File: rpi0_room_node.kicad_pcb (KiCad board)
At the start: 2 copper layers, 65 x 30 mm, 35 parts, among them IC1 DS2482-100S, J1 Raspberry Pi, J2 Conn_01x03, J3 Conn_01x03, U1 ADS1015IDGS, U2 DS18B20, U3 DS18B20

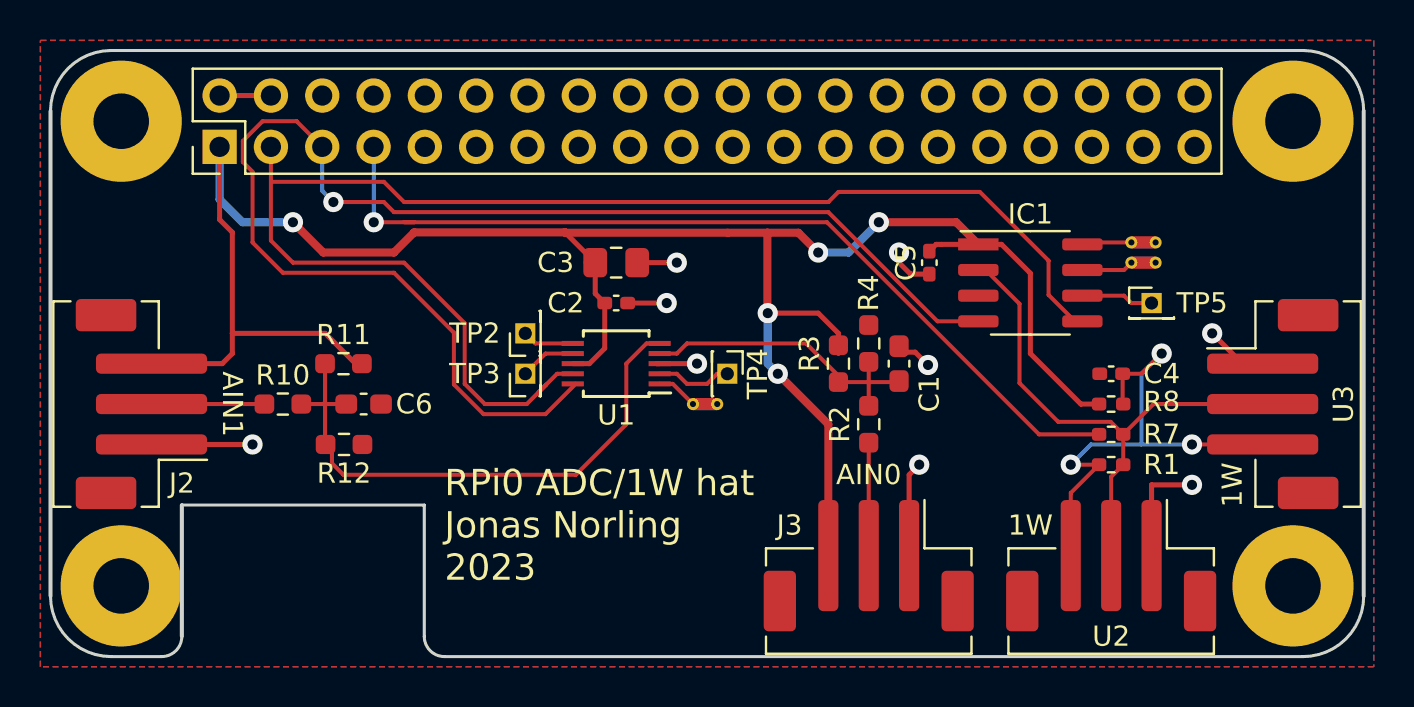
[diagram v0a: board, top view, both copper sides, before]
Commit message: Clean up, round corners
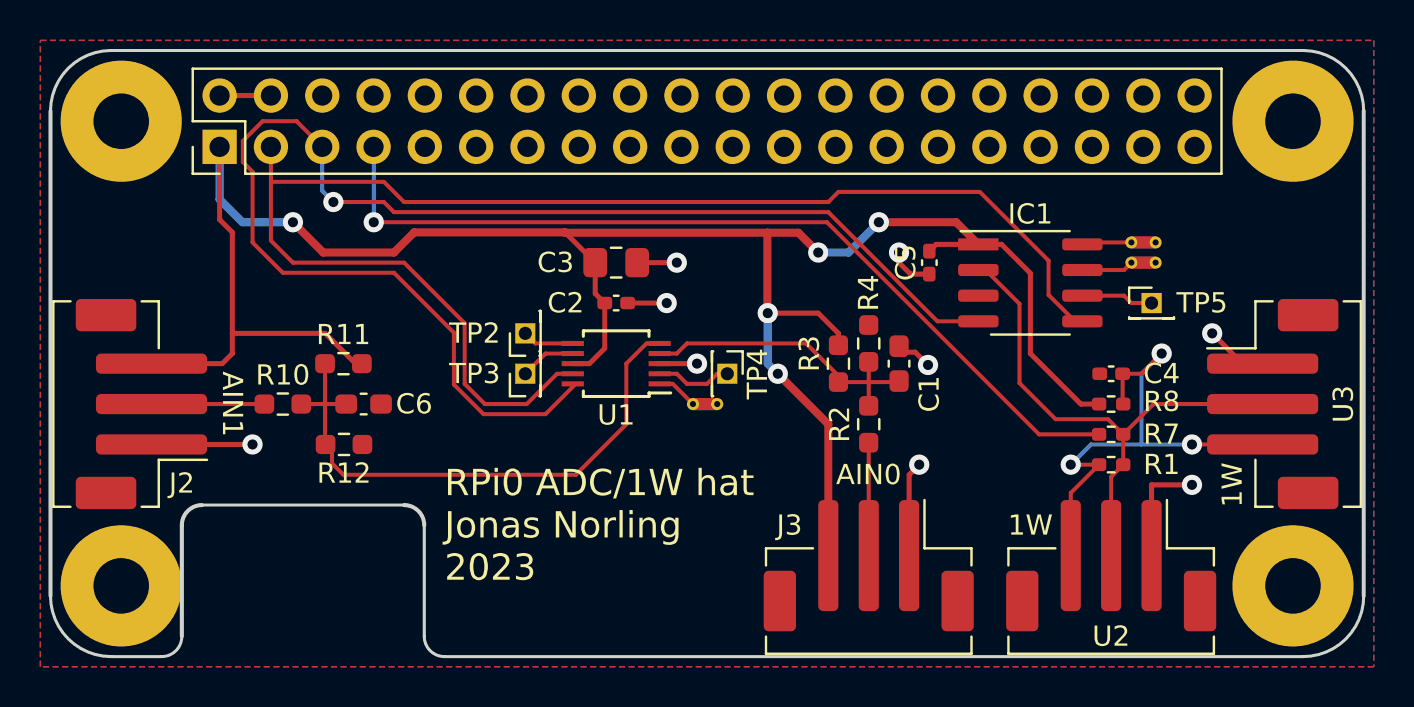
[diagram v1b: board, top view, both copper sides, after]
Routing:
- net +3.3V: track 115.4 -> 108.9 mm
- net GND: track 28.3 -> 27.2 mm
- net /SDA: track 70.2 -> 69.3 mm
- net Net-(J1-Pad7): track 44.5 -> 43.8 mm
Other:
- outline, holes or cut-outs redrawn
